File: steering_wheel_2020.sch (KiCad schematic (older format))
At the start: 38 parts, among them J1 VEHICLE, J10 Conn_01x15, J11 Conn_01x15, J12 ALT_PWR, J2 DEBUG, J3 Conn_01x15, J4 Conn_01x13, J5 Conn_01x15, J6 Conn_01x13, J7 Conn_01x15, J8 Conn_01x13, J9 Conn_01x15, U1 STM32F103R8Tx, U2 SN65HVD232, U3 LD1117S33CTR, Y1 8MHz

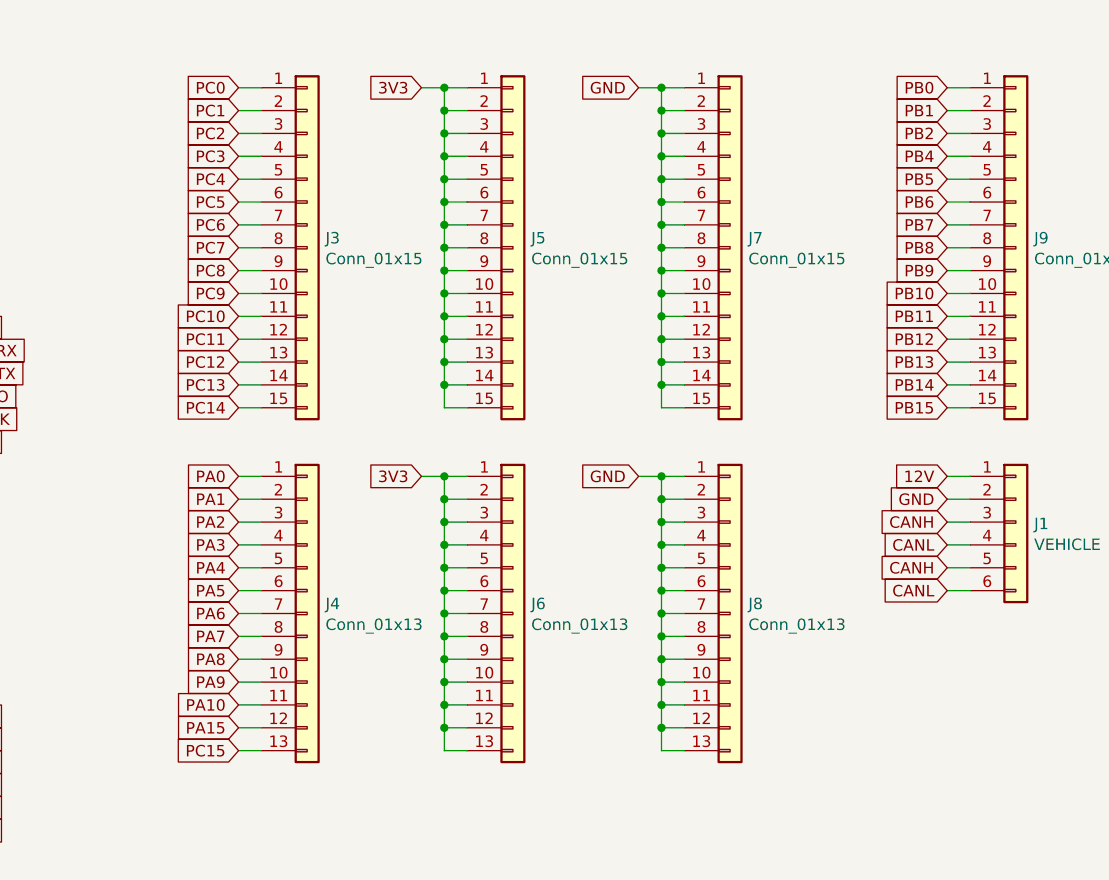
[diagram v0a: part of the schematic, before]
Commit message: begin layout
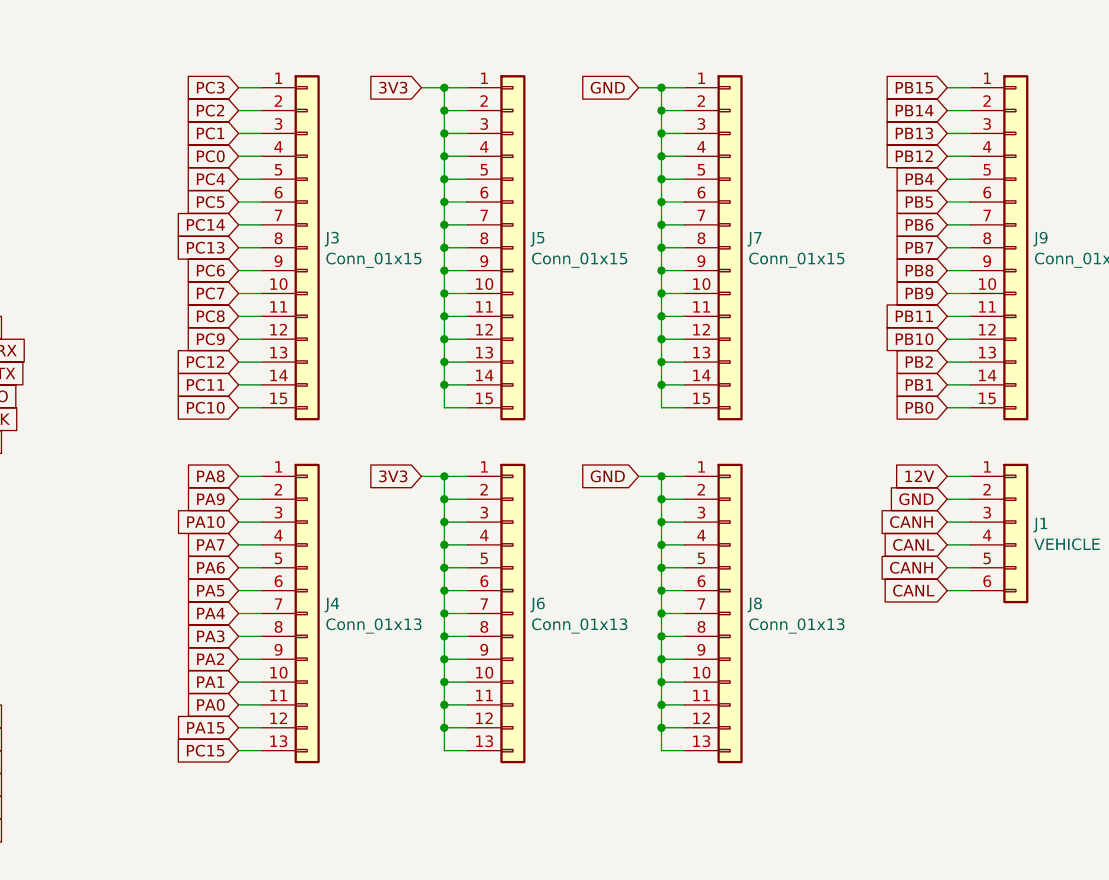
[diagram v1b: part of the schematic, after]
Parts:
- Y1: footprint Crystal:Crystal_SMD_HC49-SD -> rahulsalvi:Crystal_SMD_TXC_7A-2Pin_5x3.2mm_HandSolder
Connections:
- net PA0: now also J4.11 (Pin_11); no longer J4.1 (Pin_1)
- net PA1: now also J4.10 (Pin_10); no longer J4.2 (Pin_2)
- net PA10: now also J4.3 (Pin_3); no longer J4.11 (Pin_11)
- net PA2: now also J4.9 (Pin_9); no longer J4.3 (Pin_3)
- net PA3: now also J4.8 (Pin_8); no longer J4.4 (Pin_4)
- net PA4: now also J4.7 (Pin_7); no longer J4.5 (Pin_5)
- net PA6: now also J4.5 (Pin_5); no longer J4.7 (Pin_7)
- net PA7: now also J4.4 (Pin_4); no longer J4.8 (Pin_8)
- net PA8: now also J4.1 (Pin_1); no longer J4.9 (Pin_9)
- net PA9: now also J4.2 (Pin_2); no longer J4.10 (Pin_10)
- net PB0: now also J9.15 (Pin_15); no longer J9.1 (Pin_1)
- net PB1: now also J9.14 (Pin_14); no longer J9.2 (Pin_2)
- net PB10: now also J9.12 (Pin_12); no longer J9.10 (Pin_10)
- net PB12: now also J9.4 (Pin_4); no longer J9.12 (Pin_12)
- net PB13: now also J9.3 (Pin_3); no longer J9.13 (Pin_13)
- net PB14: now also J9.2 (Pin_2); no longer J9.14 (Pin_14)
- net PB15: now also J9.1 (Pin_1); no longer J9.15 (Pin_15)
- net PB2: now also J9.13 (Pin_13); no longer J9.3 (Pin_3)
- net PB4: now also J9.5 (Pin_5); no longer J9.4 (Pin_4)
- net PB5: now also J9.6 (Pin_6); no longer J9.5 (Pin_5)
- net PB6: now also J9.7 (Pin_7); no longer J9.6 (Pin_6)
- net PB7: now also J9.8 (Pin_8); no longer J9.7 (Pin_7)
- net PB8: now also J9.9 (Pin_9); no longer J9.8 (Pin_8)
- net PB9: now also J9.10 (Pin_10); no longer J9.9 (Pin_9)
- net PC0: now also J3.4 (Pin_4); no longer J3.1 (Pin_1)
- net PC1: now also J3.3 (Pin_3); no longer J3.2 (Pin_2)
- net PC10: now also J3.15 (Pin_15); no longer J3.11 (Pin_11)
- net PC11: now also J3.14 (Pin_14); no longer J3.12 (Pin_12)
- net PC13: now also J3.8 (Pin_8); no longer J3.14 (Pin_14)
- net PC14: now also J3.7 (Pin_7); no longer J3.15 (Pin_15)
- net PC2: now also J3.2 (Pin_2); no longer J3.3 (Pin_3)
- net PC3: now also J3.1 (Pin_1); no longer J3.4 (Pin_4)
- net PC6: now also J3.9 (Pin_9); no longer J3.7 (Pin_7)
- net PC7: now also J3.10 (Pin_10); no longer J3.8 (Pin_8)
- net PC8: now also J3.11 (Pin_11); no longer J3.9 (Pin_9)
- net PC9: now also J3.12 (Pin_12); no longer J3.10 (Pin_10)
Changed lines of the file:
@@
 EESchema Schematic File Version 4
-LIBS:steering_wheel_shield_2019-cache
+LIBS:steering_wheel_2020-cache
 EELAYER 30 0
 EELAYER END
@@
 Wire Wire Line
 	6900 1050 6900 1150
+Text GLabel 5050 1250 0    50   Input ~ 0
+PC0
+Text GLabel 5050 1150 0    50   Input ~ 0
+PC1
+Text GLabel 5050 1050 0    50   Input ~ 0
+PC2
 Text GLabel 5050 950  0    50   Input ~ 0
-PC0
-Text GLabel 5050 1050 0    50   Input ~ 0
-PC1
-Text GLabel 5050 1150 0    50   Input ~ 0
-PC2
-Text GLabel 5050 1250 0    50   Input ~ 0
 PC3
 Text GLabel 5050 1350 0    50   Input ~ 0
@@
 Text GLabel 5050 1450 0    50   Input ~ 0
 PC5
-Text GLabel 5050 1550 0    50   Input ~ 0
+Text GLabel 5050 1750 0    50   Input ~ 0
 PC6
-Text GLabel 5050 1650 0    50   Input ~ 0
+Text GLabel 5050 1850 0    50   Input ~ 0
 PC7
-Text GLabel 5050 1750 0    50   Input ~ 0
+Text GLabel 5050 1950 0    50   Input ~ 0
 PC8
-Text GLabel 5050 1850 0    50   Input ~ 0
+Text GLabel 5050 2050 0    50   Input ~ 0
 PC9
-Text GLabel 5050 1950 0    50   Input ~ 0
+Text GLabel 5050 2350 0    50   Input ~ 0
 PC10
-Text GLabel 5050 2050 0    50   Input ~ 0
+Text GLabel 5050 2250 0    50   Input ~ 0
 PC11
 Text GLabel 5050 2150 0    50   Input ~ 0
 PC12
-Text GLabel 5050 2250 0    50   Input ~ 0
+Text GLabel 5050 1650 0    50   Input ~ 0
 PC13
-Text GLabel 5050 2350 0    50   Input ~ 0
+Text GLabel 5050 1550 0    50   Input ~ 0
 PC14
 Wire Wire Line
-	5050 2350 5150 2350
-Wire Wire Line
-	5050 2250 5150 2250
-Wire Wire Line
-	5150 2150 5050 2150
-Wire Wire Line
-	5050 2050 5150 2050
-Wire Wire Line
-	5150 1950 5050 1950
-Wire Wire Line
-	5050 1850 5150 1850
-Wire Wire Line
-	5150 1750 5050 1750
-Wire Wire Line
-	5050 1650 5150 1650
-Wire Wire Line
-	5150 1550 5050 1550
-Wire Wire Line
 	5050 1450 5150 1450
 Wire Wire Line
 	5150 1350 5050 1350
-Wire Wire Line
-	5050 1250 5150 1250
-Wire Wire Line
-	5150 1150 5050 1150
-Wire Wire Line
-	5050 1050 5150 1050
-Wire Wire Line
-	5150 950  5050 950
 $Comp
 L Connector_Generic:Conn_01x15 J9
@@
 Wire Wire Line
 	10050 1050 10050 1150
-Text GLabel 8150 950  0    50   Input ~ 0
+Text GLabel 8150 2350 0    50   Input ~ 0
 PB0
-Text GLabel 8150 1050 0    50   Input ~ 0
+Text GLabel 8150 2250 0    50   Input ~ 0
 PB1
-Text GLabel 8150 1150 0    50   Input ~ 0
+Text GLabel 8150 2150 0    50   Input ~ 0
 PB2
-Text GLabel 8150 1250 0    50   Input ~ 0
+Text GLabel 8150 1350 0    50   Input ~ 0
 PB4
-Text GLabel 8150 1350 0    50   Input ~ 0
+Text GLabel 8150 1450 0    50   Input ~ 0
 PB5
-Text GLabel 8150 1450 0    50   Input ~ 0
+Text GLabel 8150 1550 0    50   Input ~ 0
 PB6
-Text GLabel 8150 1550 0    50   Input ~ 0
+Text GLabel 8150 1650 0    50   Input ~ 0
 PB7
-Text GLabel 8150 1650 0    50   Input ~ 0
+Text GLabel 8150 1750 0    50   Input ~ 0
 PB8
-Text GLabel 8150 1750 0    50   Input ~ 0
+Text GLabel 8150 1850 0    50   Input ~ 0
 PB9
-Text GLabel 8150 1850 0    50   Input ~ 0
+Text GLabel 8150 2050 0    50   Input ~ 0
 PB10
 Text GLabel 8150 1950 0    50   Input ~ 0
 PB11
-Text GLabel 8150 2050 0    50   Input ~ 0
+Text GLabel 8150 1250 0    50   Input ~ 0
 PB12
-Text GLabel 8150 2150 0    50   Input ~ 0
+Text GLabel 8150 1150 0    50   Input ~ 0
 PB13
-Text GLabel 8150 2250 0    50   Input ~ 0
+Text GLabel 8150 1050 0    50   Input ~ 0
 PB14
-Text GLabel 8150 2350 0    50   Input ~ 0
+Text GLabel 8150 950  0    50   Input ~ 0
 PB15
-Wire Wire Line
-	8150 2350 8250 2350
-Wire Wire Line
-	8150 2250 8250 2250
-Wire Wire Line
-	8150 2150 8250 2150
-Wire Wire Line
-	8150 2050 8250 2050
-Wire Wire Line
-	8150 1950 8250 1950
-Wire Wire Line
-	8150 1850 8250 1850
-Wire Wire Line
-	8150 1750 8250 1750
-Wire Wire Line
-	8150 1650 8250 1650
-Wire Wire Line
-	8150 1550 8250 1550
-Wire Wire Line
-	8150 1450 8250 1450
-Wire Wire Line
-	8150 1350 8250 1350
-Wire Wire Line
-	8150 1250 8250 1250
-Wire Wire Line
-	8150 1150 8250 1150
-Wire Wire Line
-	8150 1050 8250 1050
-Wire Wire Line
-	8150 950  8250 950
 $Comp
 L Connector_Generic:Conn_01x13 J4
@@
 	1    0    0    -1
 $EndComp
-Text GLabel 5050 2650 0    50   Input ~ 0
+Text GLabel 5050 3650 0    50   Input ~ 0
 PA0
-Text GLabel 5050 2750 0    50   Input ~ 0
+Text GLabel 5050 3550 0    50   Input ~ 0
 PA1
-Text GLabel 5050 2850 0    50   Input ~ 0
+Text GLabel 5050 3450 0    50   Input ~ 0
 PA2
-Text GLabel 5050 2950 0    50   Input ~ 0
+Text GLabel 5050 3350 0    50   Input ~ 0
 PA3
-Text GLabel 5050 3050 0    50   Input ~ 0
+Text GLabel 5050 3250 0    50   Input ~ 0
 PA4
 Text GLabel 5050 3150 0    50   Input ~ 0
 PA5
-Text GLabel 5050 3250 0    50   Input ~ 0
+Text GLabel 5050 3050 0    50   Input ~ 0
 PA6
-Text GLabel 5050 3350 0    50   Input ~ 0
+Text GLabel 5050 2950 0    50   Input ~ 0
 PA7
-Text GLabel 5050 3450 0    50   Input ~ 0
+Text GLabel 5050 2650 0    50   Input ~ 0
 PA8
-Text GLabel 5050 3550 0    50   Input ~ 0
+Text GLabel 5050 2750 0    50   Input ~ 0
 PA9
-Text GLabel 5050 3650 0    50   Input ~ 0
+Text GLabel 5050 2850 0    50   Input ~ 0
 PA10
 Text GLabel 5050 3750 0    50   Input ~ 0
@@
 Text GLabel 5050 3850 0    50   Input ~ 0
 PC15
-Wire Wire Line
-	5050 2650 5150 2650
-Wire Wire Line
-	5150 2750 5050 2750
-Wire Wire Line
-	5050 2850 5150 2850
-Wire Wire Line
-	5150 2950 5050 2950
-Wire Wire Line
-	5050 3050 5150 3050
-Wire Wire Line
-	5150 3150 5050 3150
-Wire Wire Line
-	5050 3250 5150 3250
-Wire Wire Line
-	5150 3350 5050 3350
-Wire Wire Line
-	5050 3450 5150 3450
-Wire Wire Line
-	5050 3550 5150 3550
-Wire Wire Line
-	5150 3650 5050 3650
 Wire Wire Line
 	5050 3750 5150 3750
@@
 F 0 "Y1" V 1604 2131 50  0000 L CNN
 F 1 "8MHz" V 1695 2131 50  0000 L CNN
-F 2 "Crystal:Crystal_SMD_HC49-SD" H 1650 2000 50  0001 C CNN
+F 2 "rahulsalvi:Crystal_SMD_TXC_7A-2Pin_5x3.2mm_HandSolder" H 1650 2000 50  0001 C CNN
 F 3 "~" H 1650 2000 50  0001 C CNN
 	1    1650 2000
@@
 Wire Wire Line
 	10100 3150 10200 3150
+Wire Wire Line
+	5050 1250 5150 1250
+Wire Wire Line
+	5150 1150 5050 1150
+Wire Wire Line
+	5050 1050 5150 1050
+Wire Wire Line
+	5150 950  5050 950
+Wire Wire Line
+	5050 1550 5150 1550
+Wire Wire Line
+	5150 1650 5050 1650
+Wire Wire Line
+	5050 1750 5150 1750
+Wire Wire Line
+	5150 1850 5050 1850
+Wire Wire Line
+	5050 1950 5150 1950
+Wire Wire Line
+	5150 2050 5050 2050
+Wire Wire Line
+	5150 2250 5050 2250
+Wire Wire Line
+	5050 2150 5150 2150
+Wire Wire Line
+	5050 2350 5150 2350
+Wire Wire Line
+	5050 2650 5150 2650
+Wire Wire Line
+	5050 2750 5150 2750
+Wire Wire Line
+	5050 2850 5150 2850
+Wire Wire Line
+	5050 2950 5150 2950
+Wire Wire Line
+	5050 3050 5150 3050
+Wire Wire Line
+	5050 3150 5150 3150
+Wire Wire Line
+	5050 3250 5150 3250
+Wire Wire Line
+	5050 3350 5150 3350
+Wire Wire Line
+	5050 3450 5150 3450
+Wire Wire Line
+	5050 3550 5150 3550
+Wire Wire Line
+	5050 3650 5150 3650
+Wire Wire Line
+	8150 2350 8250 2350
+Wire Wire Line
+	8150 2250 8250 2250
+Wire Wire Line
+	8150 2150 8250 2150
+Wire Wire Line
+	8150 1950 8250 1950
+Wire Wire Line
+	8150 2050 8250 2050
+Wire Wire Line
+	8150 1850 8250 1850
+Wire Wire Line
+	8150 1750 8250 1750
+Wire Wire Line
+	8150 1650 8250 1650
+Wire Wire Line
+	8150 1550 8250 1550
+Wire Wire Line
+	8150 1450 8250 1450
+Wire Wire Line
+	8150 1350 8250 1350
+Wire Wire Line
+	8150 1250 8250 1250
+Wire Wire Line
+	8150 950  8250 950
+Wire Wire Line
+	8150 1050 8250 1050
+Wire Wire Line
+	8150 1150 8250 1150
 $EndSCHEMATC
